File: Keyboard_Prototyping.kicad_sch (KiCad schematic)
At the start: 21 parts, among them J1 Conn_02x03_Odd_Even, J18 Conn_02x03_Odd_Even, J2 Conn_02x03_Odd_Even, J3 Conn_02x03_Odd_Even, J4 Conn_02x03_Odd_Even, J5 Conn_01x08, J6 Conn_02x03_Odd_Even, J7 Conn_02x03_Odd_Even, J8 Conn_02x03_Odd_Even, SW1 A, SW2 C, SW3 B, SW4 D

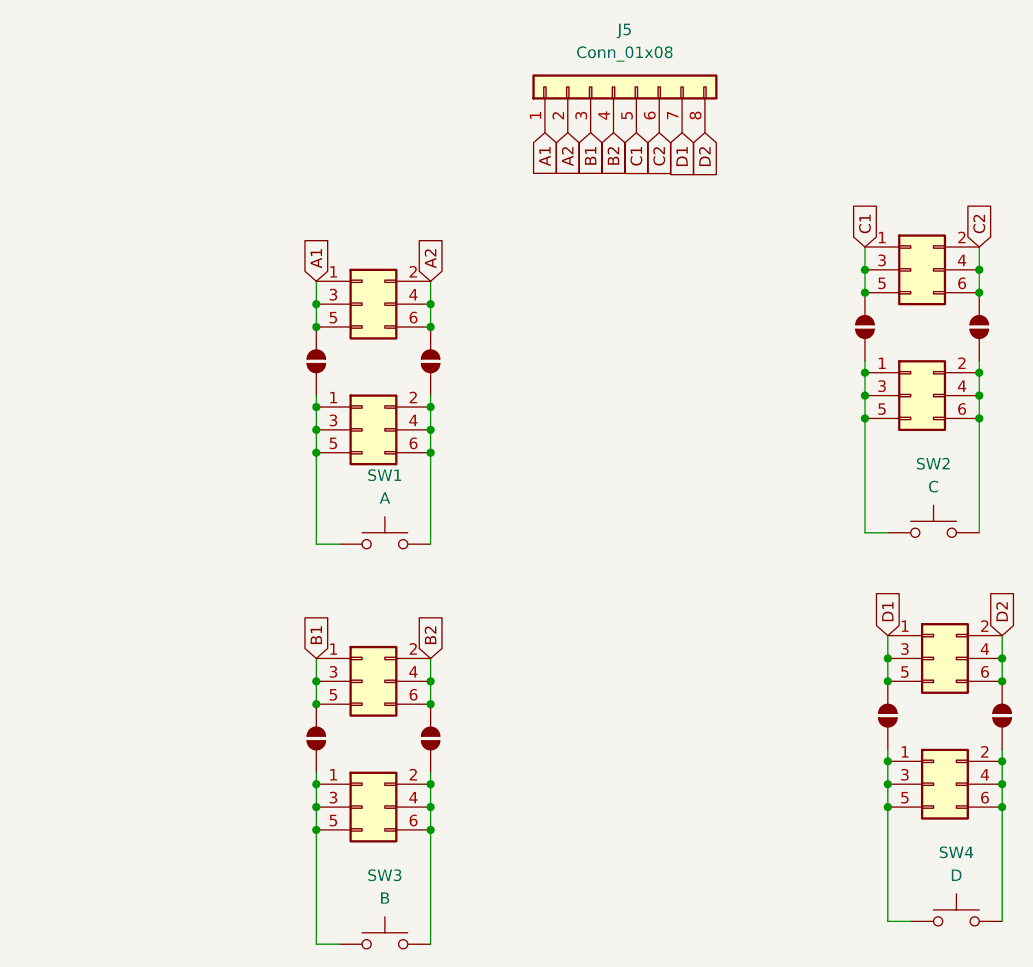
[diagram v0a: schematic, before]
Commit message: Generated fabrication files
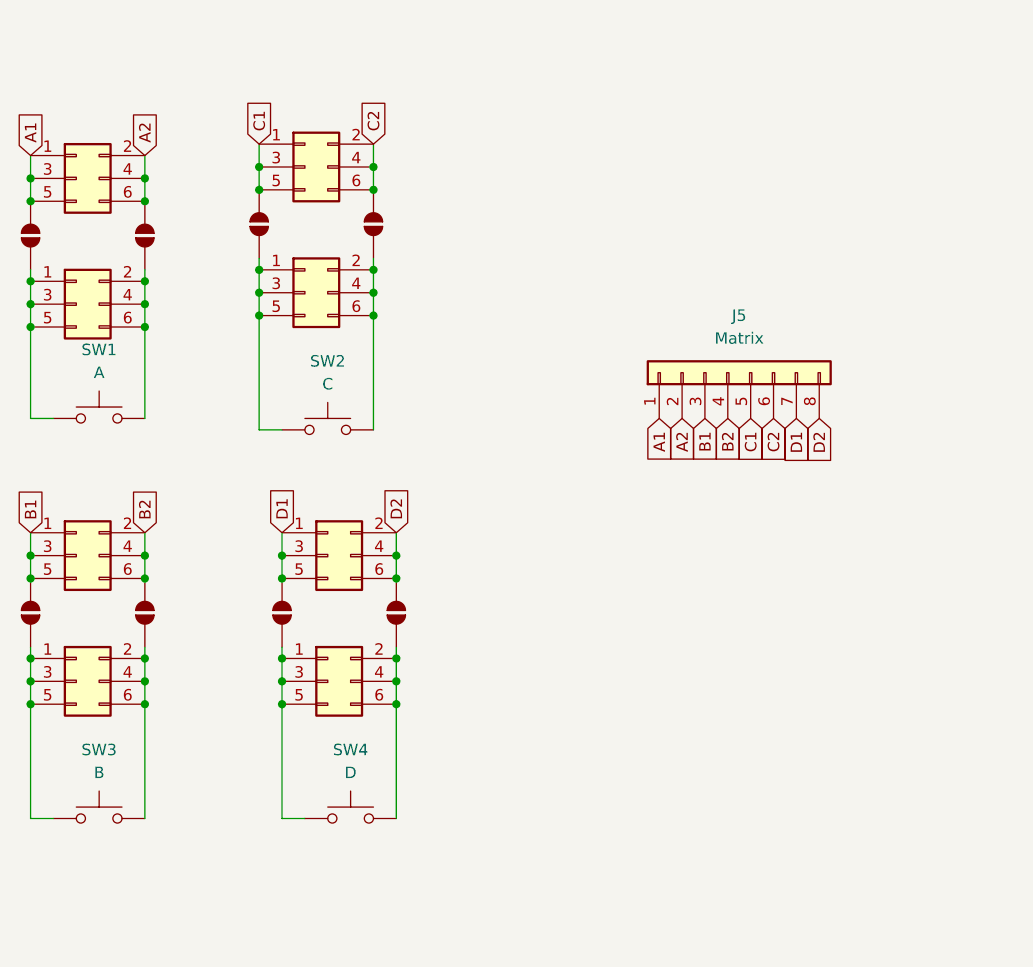
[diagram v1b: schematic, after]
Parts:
- J5: value Conn_01x08 -> Matrix
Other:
- company: (none) -> Brett Hallen
- title: (none) -> Keyboard Prototyping Board
- moved on the sheet: J5, SW1, SW2, SW3, SW4
